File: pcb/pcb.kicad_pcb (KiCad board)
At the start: 2 copper layers, 136 x 91.7 mm, 56 parts, among them J1 BATT, J2 BATT, SW1 SW_SPST, SW10 SW_SPST, SW11 SW_SPST, SW12 SW_SPST, SW13 SW_SPST, SW14 SW_SPST, SW15 SW_SPST, SW16 SW_SPST, SW17 SW_SPST, SW18 SW_SPST, SW19 SW_SPST, SW2 SW_SPST, SW20 SW_SPST, SW21 SW_SPST, SW3 SW_SPST, SW4 SW_SPST, SW5 SW_SPST, SW6 SW_SPST, SW7 SW_SPST, SW8 SW_SPST, SW9 SW_SPST, U1 XIAO_nRF52840

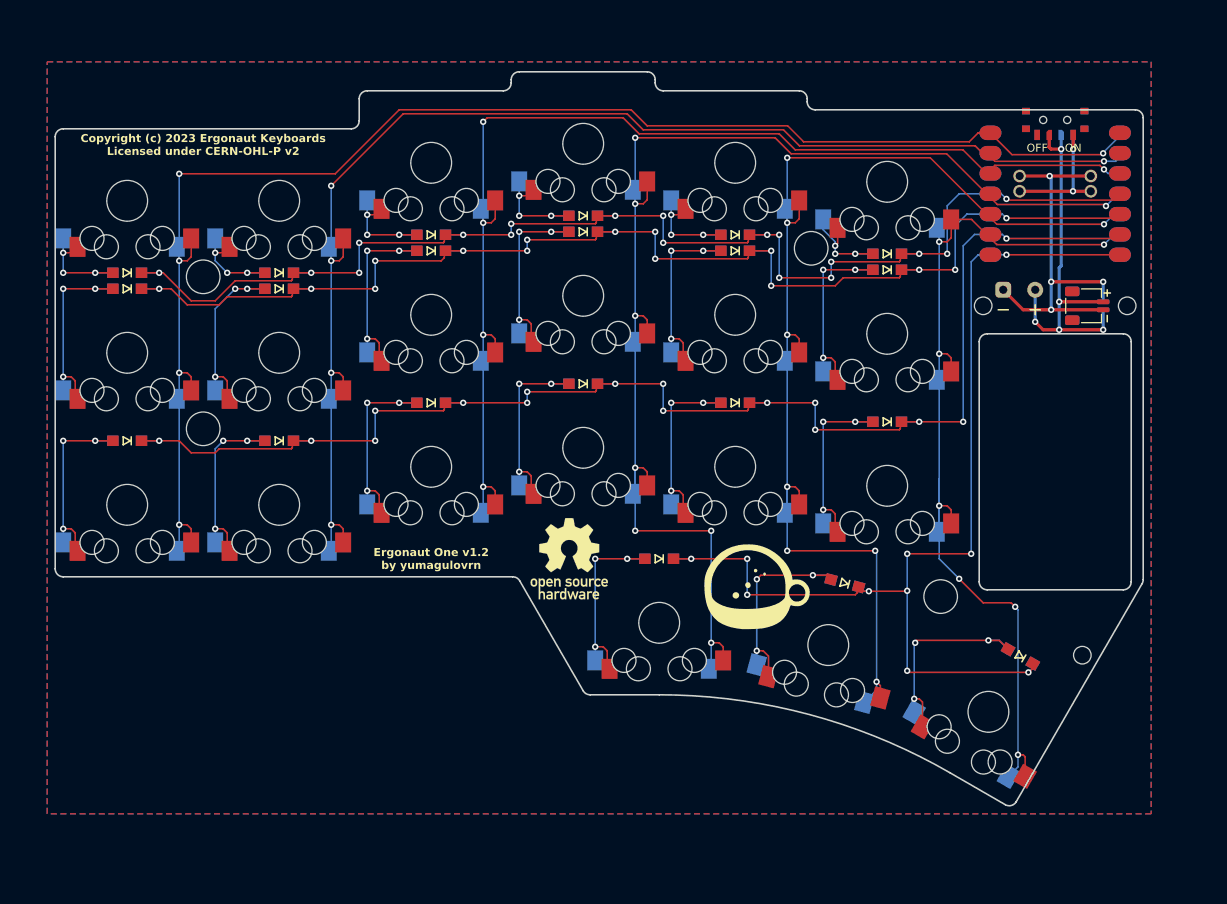
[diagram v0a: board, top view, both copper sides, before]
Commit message: init changes
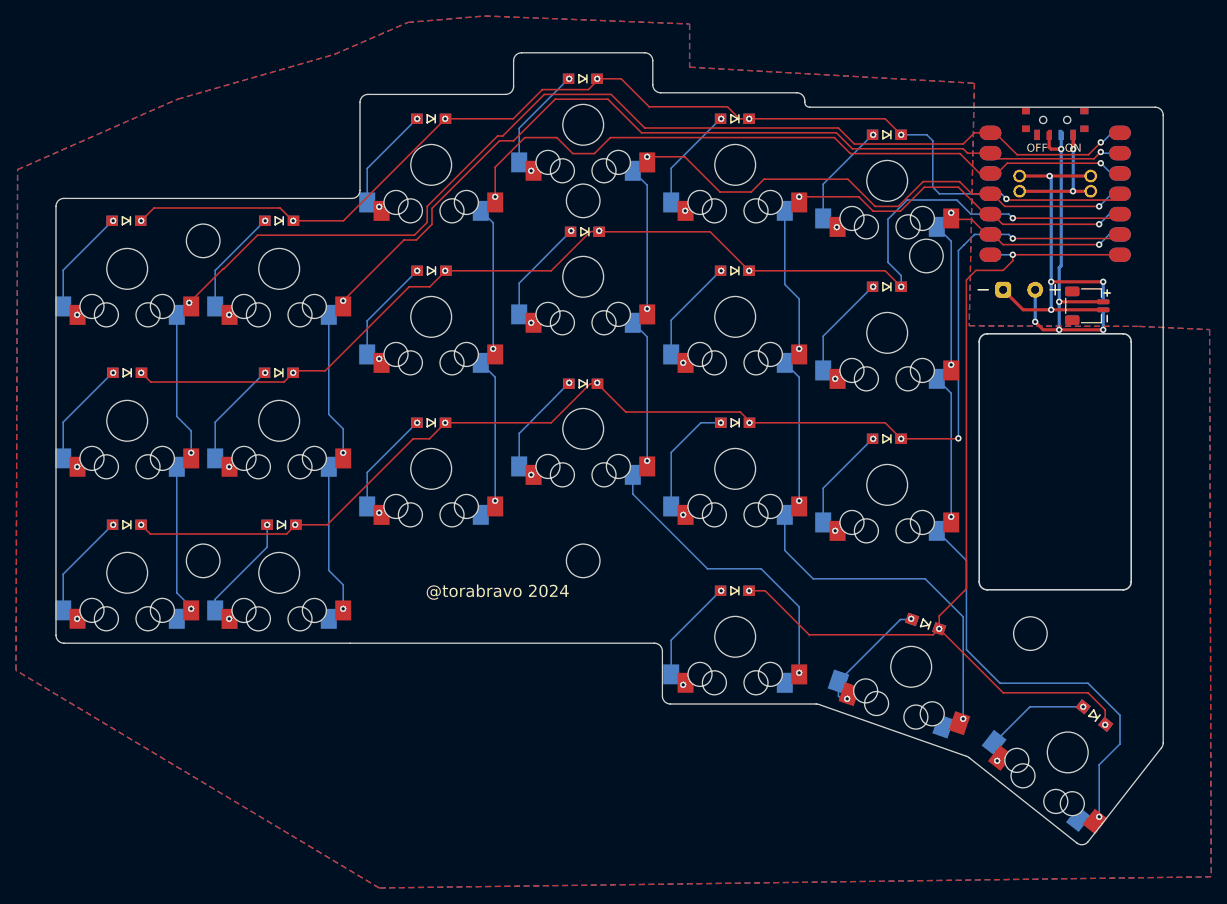
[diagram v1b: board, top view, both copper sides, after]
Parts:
- removed G*** (x2): LOGO, one:OSHW-logo
- removed G***: LOGO, one:en_logo
- removed H6, H7, H8: StandoffHole, one:Hole_2.2mm
- added H3: MountingHole, one:Hole_4.2mm, F.Cu at (141.5, 112.0)
- added H3: MountingHole, one:Hole_4.2mm, F.Cu at (141.5, 67.0)
- moved D4 17.1 mm to (141.5, 51.7)
- moved H2 16.5 mm to (94.0, 112.0)
- moved D6 14.9 mm to (179.5, 58.7)
- moved D5 14.5 mm to (160.5, 56.7)
- moved D3 14.5 mm to (122.5, 56.7)
- moved H3 14.4 mm to (184.4, 73.9)
- moved ? 12.1 mm to (197.4, 121.1)
- moved D21 11.9 mm to (205.4, 131.3), turned to 142 degrees
- moved D20 11.3 mm to (184.3, 119.9), turned to 161 degrees
- moved SW21 11.1 mm to (202.1, 135.9), turned to -38 degrees
- moved SW20 10.7 mm to (182.5, 125.2), turned to -19 degrees
- moved D14 10.5 mm to (103.8, 107.5)
- moved D13 10.5 mm to (84.5, 107.5)
- moved D8 10.5 mm to (103.5, 88.5)
- moved D7 10.5 mm to (84.5, 88.5)
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- renumbered H4 to ?
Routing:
- net R0: track 165.5 -> 141.9 mm, vias 18 -> 7
- net R2: track 175.6 -> 159.0 mm, vias 16 -> 8
- net C2: track 145.9 -> 131.8 mm, vias 5 -> 4
- net R1: track 161.3 -> 147.2 mm, vias 15 -> 7
- net Net-(D21-A): track 28.2 -> 15.4 mm, vias 3 -> 2
- net R3: track 134.9 -> 122.9 mm, vias 10 -> 4
- net Net-(D20-A): track 27.2 -> 15.6 mm, vias 3 -> 2
- net C3: track 160.6 -> 149.9 mm, vias 8 -> 5
- net Net-(D9-A): track 25.2 -> 14.8 mm, vias 3 -> 2
- net Net-(D15-A): track 25.2 -> 15.0 mm, vias 3 -> 2
- net Net-(D18-A): track 25.2 -> 15.2 mm, vias 3 -> 2
- net Net-(D12-A): track 25.2 -> 15.2 mm, vias 3 -> 2
- net Net-(D11-A): track 25.2 -> 15.2 mm, vias 3 -> 2
- net C4: track 144.3 -> 134.4 mm, vias 8 -> 5
- net Net-(D19-A): track 25.2 -> 15.3 mm, vias 3 -> 2
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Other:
- board size 136 x 91.7 mm -> 138.4 x 99 mm
- board text added: "@torabravo 2024"
- board text removed: "Copyright (c) 2023 Ergonaut Keyboards Licensed under CERN-OHL-P v2"
- board text removed: "Ergonaut One v1.2 by yumagulovrn"
